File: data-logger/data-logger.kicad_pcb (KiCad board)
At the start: 2 copper layers, 30 parts, among them J1 MPT-0,5-2-2.54, J2 MPT-0,5-2-2.54, J3 MPT-0,5-2-2.54, J4 SM04B-GHS-TB, J5 SM04B-GHS-TB, J6 SM04B-GHS-TB, J7 DM3D-SF, J8 SM04B-GHS-TB, J9 Conn_01x04, U3 MAX31855KASA, U4 MAX31855KASA, U5 MAX31855KASA

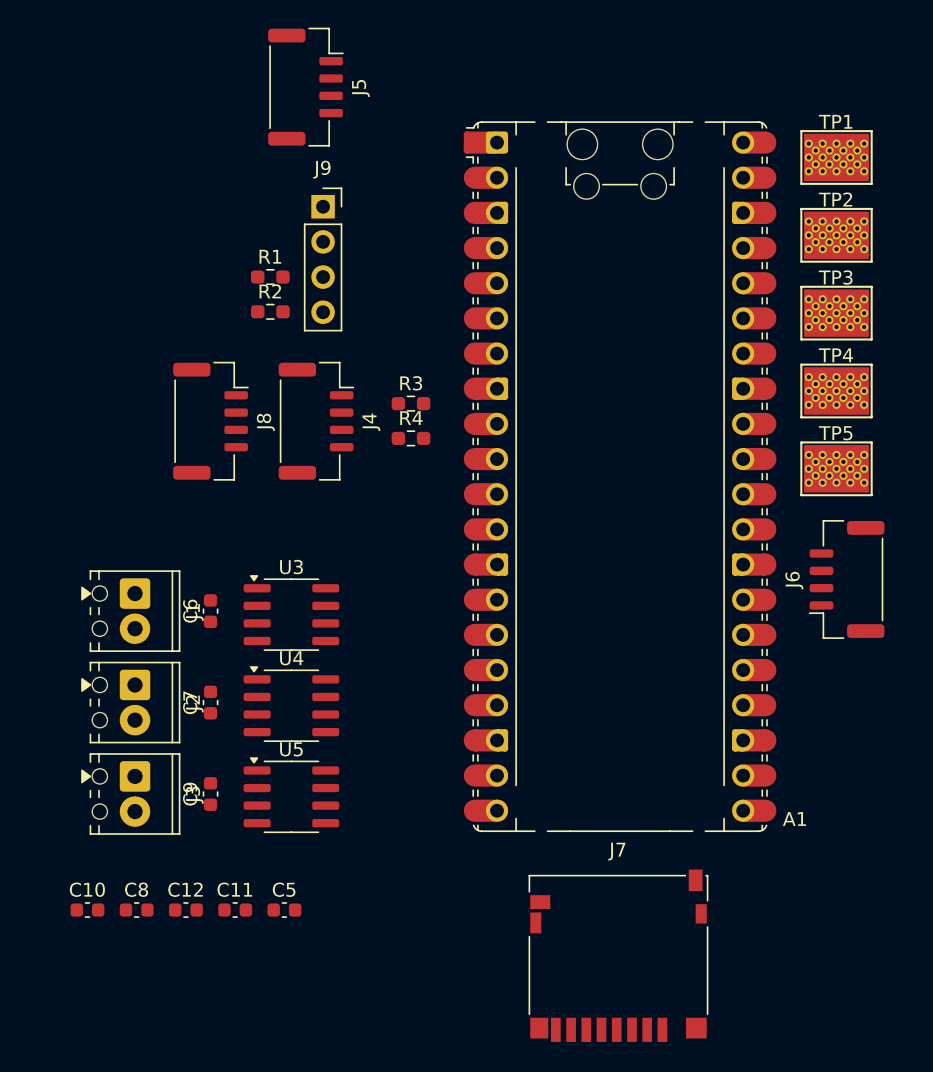
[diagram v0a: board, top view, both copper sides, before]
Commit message: layout
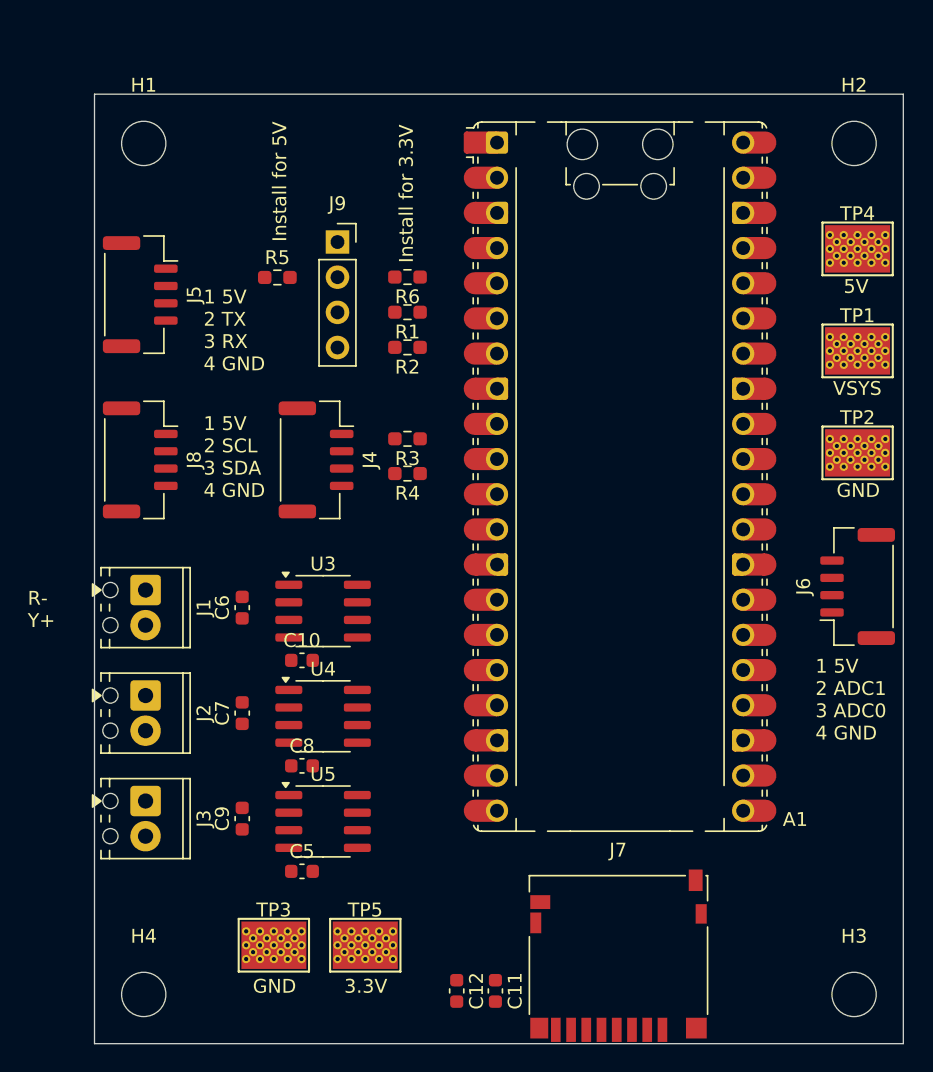
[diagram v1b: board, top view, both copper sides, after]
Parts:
- added H1: MountingHole, MountingHole:MountingHole_3.2mm_M3, F.Cu at (105.2, 74.7)
- added H2: MountingHole, MountingHole:MountingHole_3.2mm_M3, F.Cu at (156.5, 74.7)
- added H3: MountingHole, MountingHole:MountingHole_3.2mm_M3, F.Cu at (156.5, 136.1)
- added H4: MountingHole, MountingHole:MountingHole_3.2mm_M3, F.Cu at (105.2, 136.1)
- added R5: 0, Resistor_SMD:R_0603_1608Metric_Pad0.98x0.95mm_HandSolder, F.Cu at (114.8, 84.4)
- added R6: 0, Resistor_SMD:R_0603_1608Metric_Pad0.98x0.95mm_HandSolder, F.Cu at (124.2, 84.3)
- moved TP3 61.1 mm to (114.6, 132.6)
- moved TP5 48.4 mm to (121.2, 132.6)
- moved C10 23.8 mm to (116.6, 112.0)
- moved C12 20.4 mm to (127.8, 135.9), turned to -90 degrees
- moved C11 19.7 mm to (130.6, 135.9), turned to -90 degrees
- moved J5 19.2 mm to (104.9, 85.6)
- moved C8 15.8 mm to (116.6, 119.6)
- moved TP2 15.8 mm to (156.7, 97.0)
- moved TP1 14.1 mm to (156.7, 89.7)
- moved TP4 10.4 mm to (156.7, 82.3)
- moved R2 10.2 mm to (124.2, 89.4), turned to 180 degrees
- moved R1 10.2 mm to (124.2, 86.9), turned to 180 degrees
- moved J8 5.80 mm to (104.9, 97.5)
- moved C5 3.07 mm to (116.6, 127.3)
- moved C9 2.90 mm to (112.3, 123.4)
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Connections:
- J9 pad 2: +3.3V -> Net-(J9-Pin_2)
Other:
- board outline added: 58.4 x 68.6 mm
- board text added: "1 5V 2 ADC1 3 ADC0 4 GND"
- board text added: "1 5V 2 SCL 3 SDA 4 GND"
- board text added: "1 5V 2 TX 3 RX 4 GND"
- board text added: "3.3V"
- board text added: "5V"
- board text added: "GND"
- board text added: "Install for 3.3V"
- board text added: "Install for 5V"
- board text added: "R- Y+"
- board text added: "VSYS"
